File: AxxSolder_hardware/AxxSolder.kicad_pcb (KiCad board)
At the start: 2 copper layers, 39 x 82.5 mm, 128 parts, among them IC1 OPA2387DSGT, IC2 STM32F303CCT6TR, IC3 TPS54302DDCR, IC4 STUSB4500QTR, IC5 LTC4440AHMS8E, IC6 MAX16171ATA_VY+T, J1 USB4110-GF-A, J2 691243110009, J3 Conn_01x05_Socket, J4 Conn_01x02_Pin, Q1 STL9P3LLH6, Q2 2N7002NXAKR, Q3 STL10N3LLH5, U3 PEC11J-9220F-S0015, U4 BSC014N04LS, Y1 NX2016SA-32M-EXS00A-CS06465

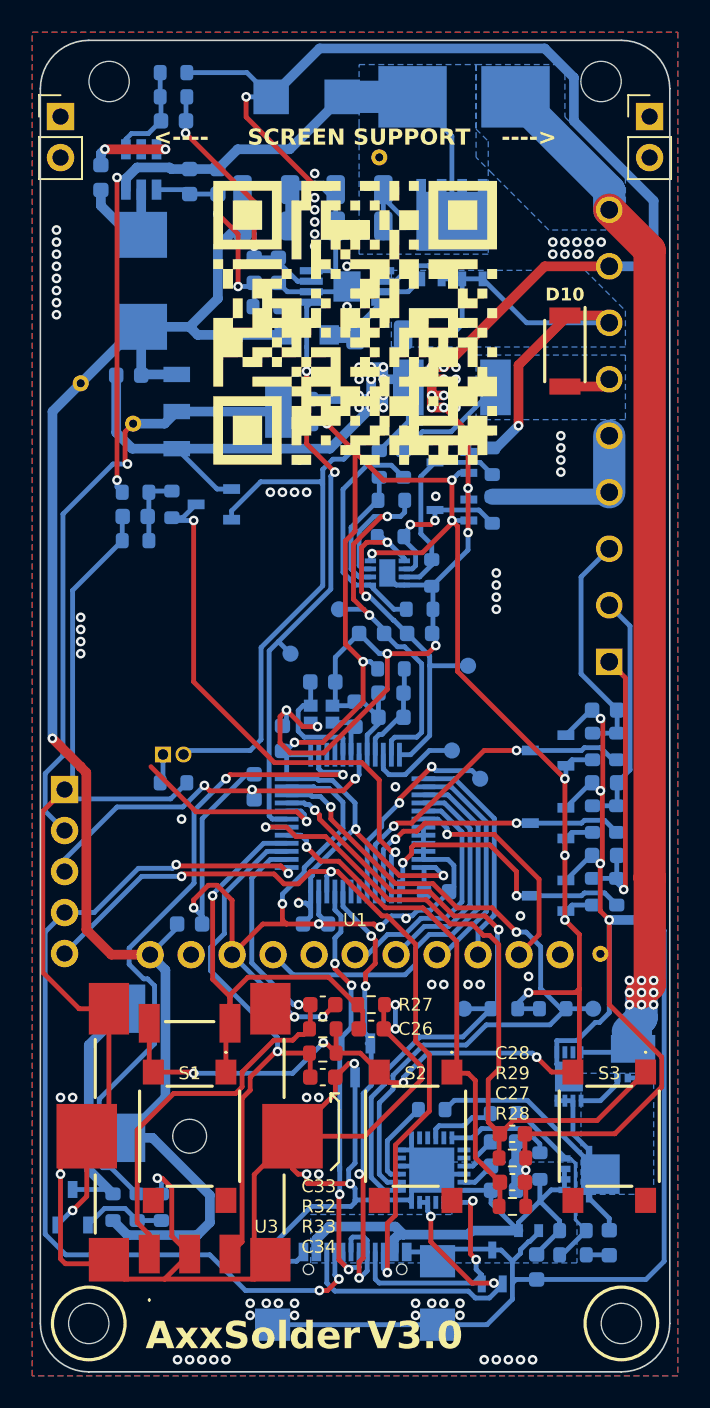
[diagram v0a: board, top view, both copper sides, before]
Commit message: updates in hardware and software
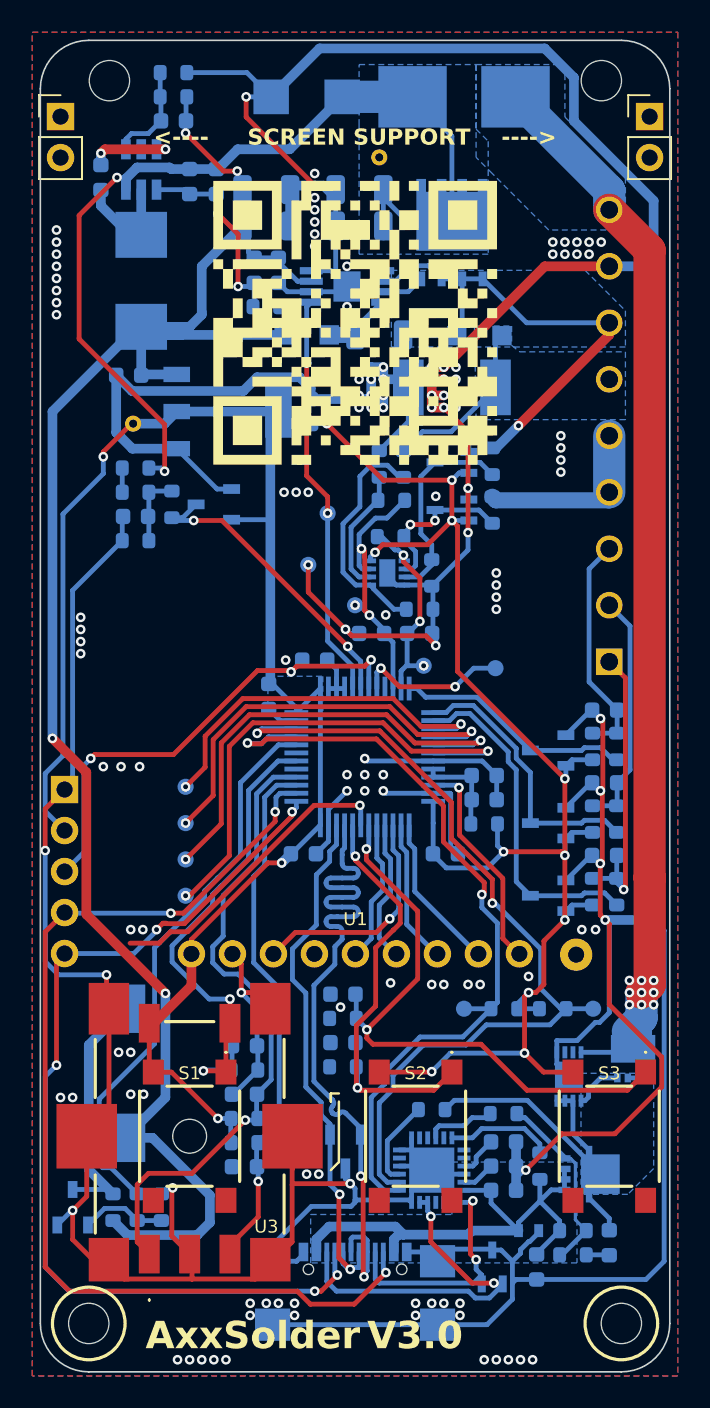
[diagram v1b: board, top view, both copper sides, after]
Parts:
- removed C12, C3: 10p, Capacitor_SMD:C_0603_1608Metric
- removed C15: 10u, Capacitor_SMD:C_0603_1608Metric
- removed D10: PMEG10030ELPX, footprints:SODFL4725X110N
- removed IC2: STM32F303CCT6TR, footprints:QFP50P900X900X160-48N
- removed J4: Conn_01x02_Pin, Connector_PinHeader_1.27mm:PinHeader_1x02_P1.27mm_Vertical
- removed R40: 4k7, Resistor_SMD:R_0603_1608Metric
- removed Y1: NX2016SA-32M-EXS00A-CS06465, footprints:NX2016SA32MEXS00ACS06465
- added D13: PMEG6020ER, footprints:PMEG6020ER115, B.Cu at (188.2, 85.8)
- added IC7: STM32G431CBT6, footprints:QFP50P900X900X160-48N, B.Cu at (181.1, 111.9)
- added R41: 22k, Resistor_SMD:R_0603_1608Metric, B.Cu at (166.9, 94.0)
- added TP13: DIAG_TP, TestPoint:TestPoint_Pad_D1.0mm, B.Cu at (170.0, 120.5)
- added TP14: TC_TP, TestPoint:TestPoint_Pad_D1.0mm, B.Cu at (177.6, 100.0)
- added TP15: DIAG_TP, TestPoint:TestPoint_Pad_D1.0mm, B.Cu at (189.2, 106.4)
- C16, C17, C18: value 1u -> 10u
- C26, C27, C28, C33, C34, R27, R28, R29, R32, R33: moved to B.Cu
- R10: value 13k3 -> 22k
- R13, R15: value 1k -> 1k5
- R21: value 47k -> 22k
- R6: value 100k -> 220k
- TP1: value VDD_TP -> DIAG_TP; footprint TestPoint:TestPoint_THTPad_D1.0mm_Drill0.5mm -> TestPoint:TestPoint_Pad_D1.0mm
- TP6: footprint TestPoint:TestPoint_THTPad_D1.0mm_Drill0.5mm -> TestPoint:TestPoint_THTPad_D2.0mm_Drill1.0mm
- moved TP1 30.2 mm to (170.0, 118.2)
- moved TP10 18.5 mm to (170.0, 116.0)
- moved TP9 16.7 mm to (170.0, 113.8)
- moved C27 13.6 mm to (179.8, 129.6), turned to 180 degrees
- moved C28 13.6 mm to (179.8, 126.6), turned to 180 degrees
- moved R28 13.6 mm to (179.8, 131.1), turned to 180 degrees
- moved R29 13.6 mm to (179.8, 128.1), turned to 180 degrees
- moved FB1 11.2 mm to (188.5, 116.0), turned to 0 degrees
- moved TP8 9.00 mm to (178.8, 96.8)
- moved R27 8.83 mm to (173.7, 131.3)
- moved C25 8.78 mm to (188.5, 114.5), turned to 0 degrees
- moved C14 8.70 mm to (178.0, 105.9), turned to 180 degrees
- moved C26 7.92 mm to (173.7, 129.8)
- moved C33 7.37 mm to (173.7, 132.8), turned to 180 degrees
- moved R32 7.37 mm to (173.7, 134.3), turned to 180 degrees
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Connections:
- net /Current renamed /CURRENT
- net /VDD_inp renamed /VBUS_IN
- C1 pad 2: +5V -> +6V
- C36 pad 1: +5V -> +6V
- C37 pad 1: +5V -> +6V
- C7 pad 2: +5V -> +6V
- C8 pad 2: +5V -> +6V
- C9 pad 2: +5V -> +6V
- D9 pad 2: +5V -> +6V
- IC5 pad 3: +5V -> +6V
- J1 pad A8: /SWCLK -> /SWDIO
- J1 pad B8: /SWDIO -> /SWCLK
- L1 pad 2: +5V -> +6V
- LS1 pad 2: +5V -> +6V
- PS1 pad 3: +5V -> +6V
- R20 pad 1: +5V -> +6V
- R21 pad 1: VDD -> Net-(R21-Pad1)
- R6 pad 1: +5V -> +6V
- TP1 pad 1: +5V -> /USR3
- U1 pad 2: unconnected-(U1-NC-Pad2) -> +3.3V
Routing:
- net +5V: track 123.6 -> 0.00 mm, vias 3 -> 0
- net +6V: track 0.00 -> 117.5 mm, vias 0 -> 4
- net GND: track 601.3 -> 504.8 mm, vias 132 -> 137
- net +3.3V: track 231.8 -> 197.4 mm, vias 19 -> 14
- net /USR4: track 0.00 -> 31.3 mm, vias 0 -> 2
- net /USR3: track 0.00 -> 28.8 mm, vias 0 -> 2
- net /USART_TX: track 0.00 -> 19.0 mm, vias 0 -> 1
- net /USR1: track 5.90 -> 23.1 mm, vias 0 -> 2
- net /VBUS_IN: track 34.8 -> 19.0 mm
- net /USB_D-: track 30.2 -> 45.0 mm, vias 4 -> 2
- net /BOOT0: track 14.6 -> 0.00 mm, vias 1 -> 0
- net /USR2: track 12.7 -> 26.0 mm
- net /Heater: track 38.7 -> 27.3 mm
- net /CURRENT: track 28.4 -> 17.2 mm, vias 2 -> 3
- net /SPI_SCK: track 24.8 -> 14.3 mm, vias 0 -> 1
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- added copper zone on B.Cu, net +3.3V
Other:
- board text added: "IO1"
- board text added: "IO2"
- board text added: "IO3"
- board text added: "IO4"
- board text added: "USBC-PD"
- board text removed: "5V"
- board text removed: "BOOT0"
- board text removed: "USBC-PD 100W"
- board text removed: "USR1"
- board text removed: "USR2"
- board text removed: "V3.1"
